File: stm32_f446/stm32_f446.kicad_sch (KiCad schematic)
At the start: 35 parts, among them J1 USB_B_Mini, J10 right_engine, J2 UART, J3 I2C, J4 SPI, J5 L293D_right, J6 L293D_left, J9 left_engine, SW1 SW_Push, SW2 SW_SPDT, U1 STM32F446RETx, U2 AMS1117-3.3, Y2 16MHz

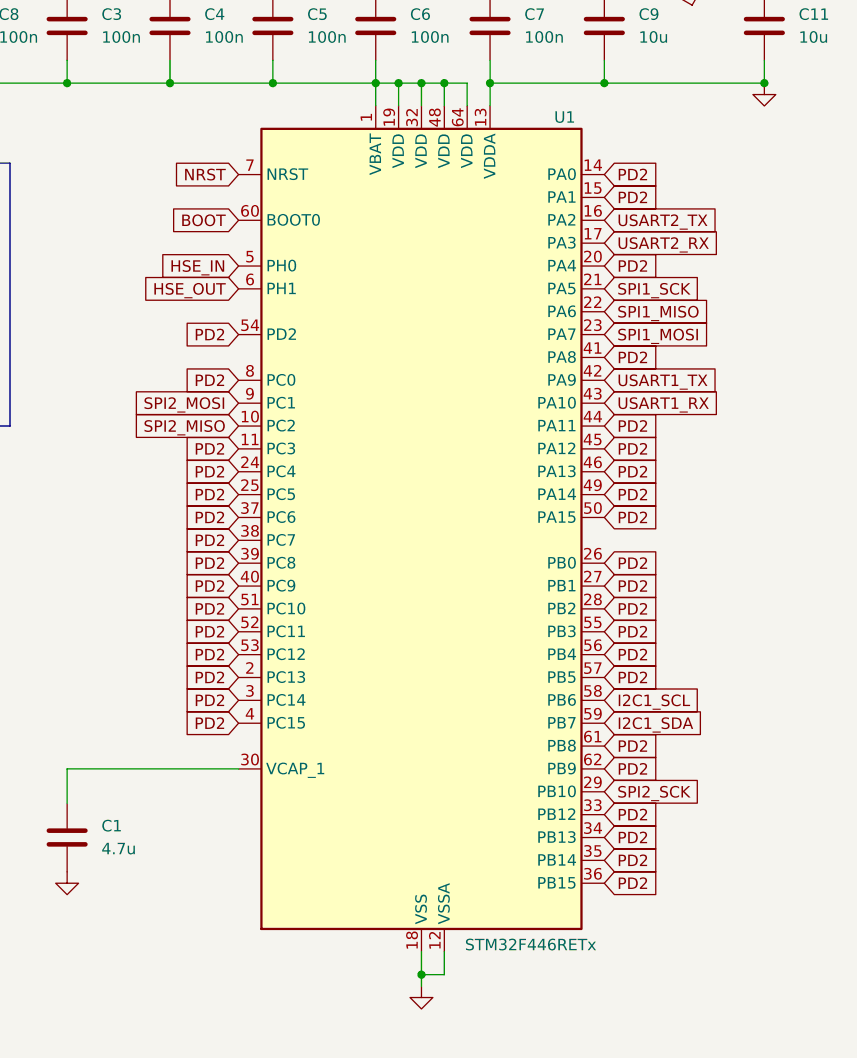
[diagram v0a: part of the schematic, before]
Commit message: Cleaning in files part 1
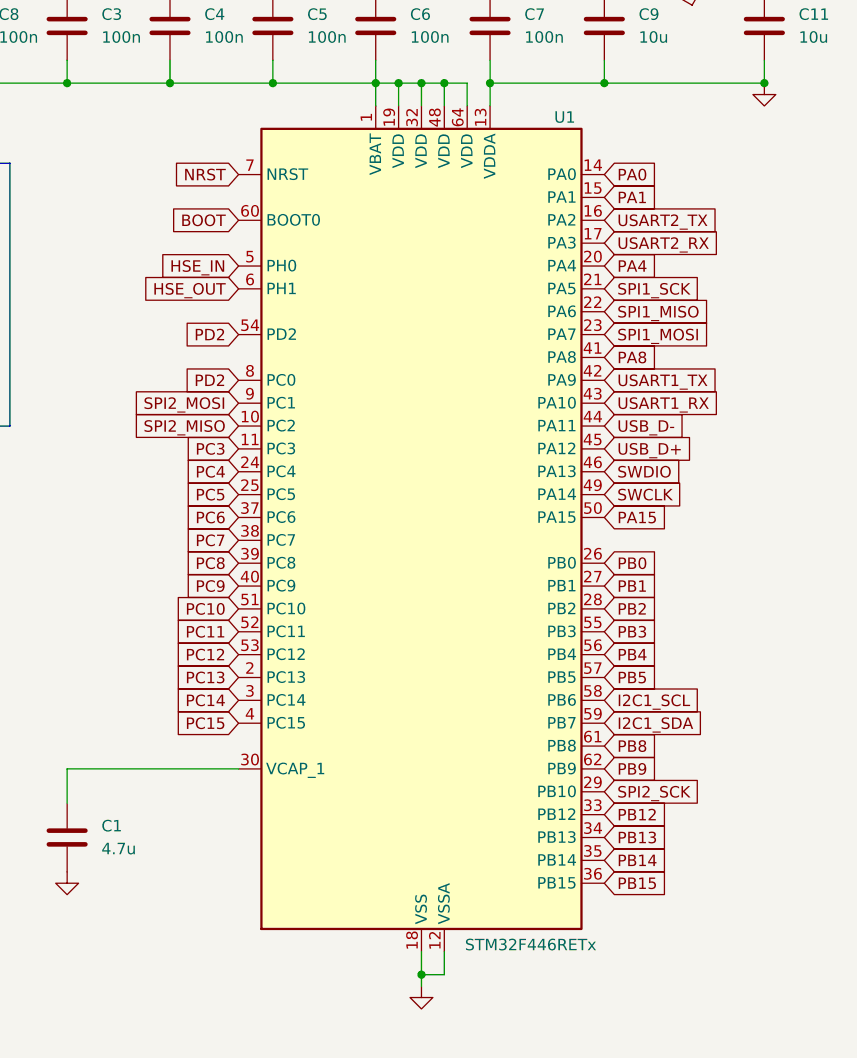
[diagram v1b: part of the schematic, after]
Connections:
- net PD2: no longer U1.11 (PC3), U1.14 (PA0), U1.15 (PA1), U1.2 (PC13), U1.20 (PA4), U1.24 (PC4), U1.25 (PC5), U1.26 (PB0), U1.27 (PB1), U1.28 (PB2), U1.3 (PC14), U1.33 (PB12), U1.34 (PB13), U1.35 (PB14), U1.36 (PB15), U1.37 (PC6), U1.38 (PC7), U1.39 (PC8), U1.4 (PC15), U1.40 (PC9), U1.41 (PA8), U1.44 (PA11), U1.45 (PA12), U1.46 (PA13), U1.49 (PA14), U1.50 (PA15), U1.51 (PC10), U1.52 (PC11), U1.53 (PC12), U1.55 (PB3), U1.56 (PB4), U1.57 (PB5), U1.61 (PB8), U1.62 (PB9)
- net USB_D+: now also U1.45 (PA12)
- net USB_D-: now also U1.44 (PA11)
- new net PA0: U1.14 (PA0)
- new net PA1: U1.15 (PA1)
- new net PA15: U1.50 (PA15)
- new net PA4: U1.20 (PA4)
- new net PA8: U1.41 (PA8)
- new net PB0: U1.26 (PB0)
- new net PB1: U1.27 (PB1)
- new net PB12: U1.33 (PB12)
- new net PB13: U1.34 (PB13)
- new net PB14: U1.35 (PB14)
- new net PB15: U1.36 (PB15)
- new net PB2: U1.28 (PB2)
- new net PB3: U1.55 (PB3)
- new net PB4: U1.56 (PB4)
- new net PB5: U1.57 (PB5)
- new net PB8: U1.61 (PB8)
- new net PB9: U1.62 (PB9)
- new net PC10: U1.51 (PC10)
- new net PC11: U1.52 (PC11)
- new net PC12: U1.53 (PC12)
- new net PC13: U1.2 (PC13)
- new net PC14: U1.3 (PC14)
- new net PC15: U1.4 (PC15)
- new net PC3: U1.11 (PC3)
- new net PC4: U1.24 (PC4)
- new net PC5: U1.25 (PC5)
- new net PC6: U1.37 (PC6)
- new net PC7: U1.38 (PC7)
- new net PC8: U1.39 (PC8)
- new net PC9: U1.40 (PC9)
- new net SWCLK: U1.49 (PA14)
- new net SWDIO: U1.46 (PA13)
